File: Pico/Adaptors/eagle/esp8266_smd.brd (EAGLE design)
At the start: 29.5 x 17.8 mm, 3 parts

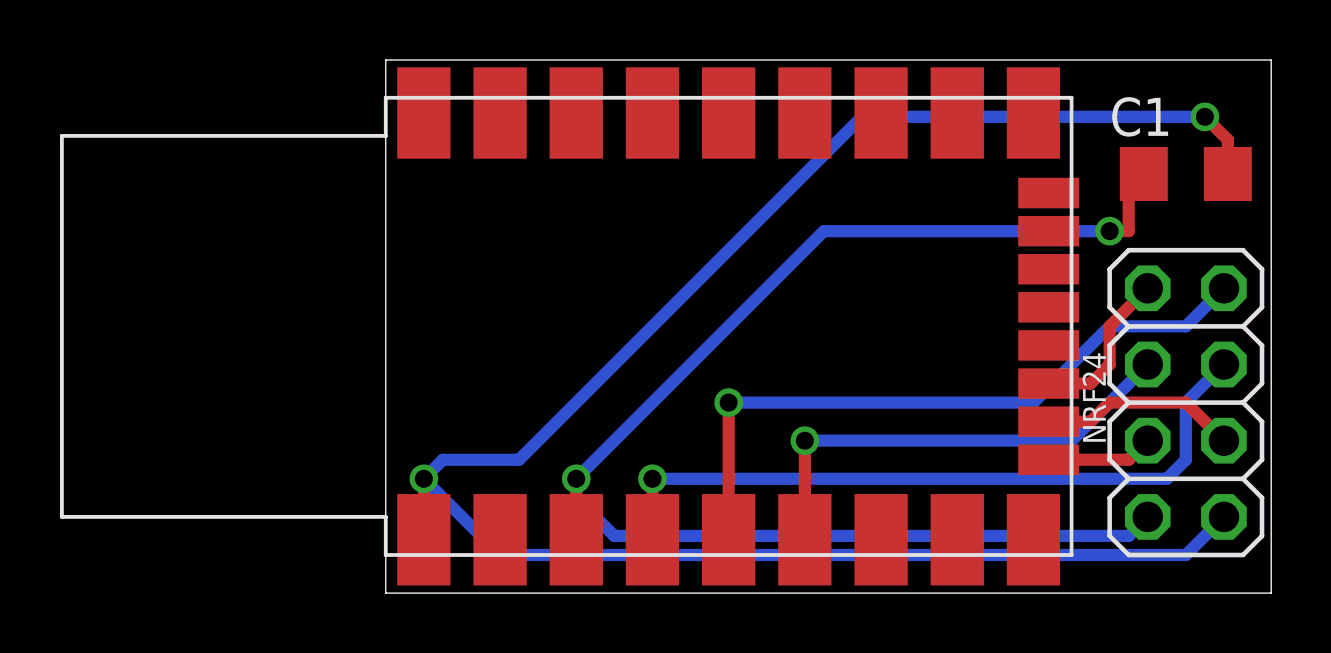
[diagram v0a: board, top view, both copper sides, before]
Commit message: tweaking
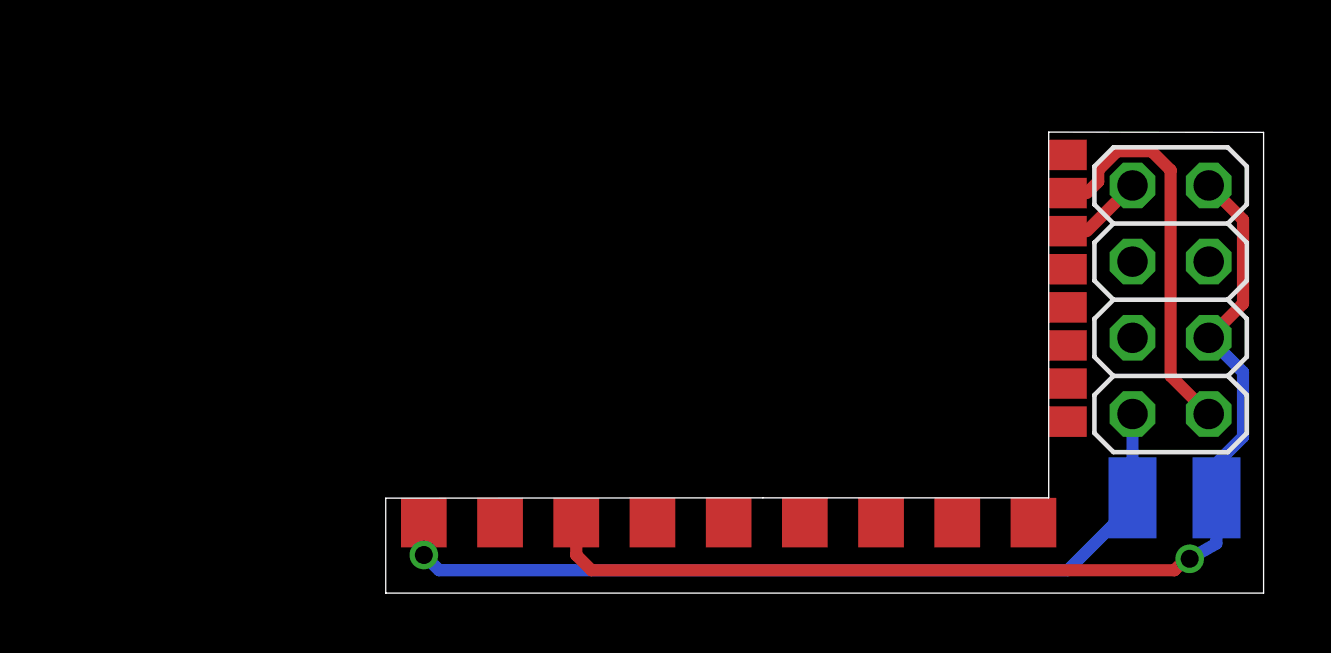
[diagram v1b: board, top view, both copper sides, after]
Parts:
- removed NRF24: (no value), pinhead:2X04
- removed U$1: ESPRUINO_PICO_SMDONLY, espruino_pico:ESPRUINO_PICO_SMDONLY
- added ESP8266: (no value), pinhead:2X04
- C1: device rcl:C1206 -> rcl:C1210
- moved C1 10.8 mm to (26.3, 3.17), flipped to the bottom
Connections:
- removed net N$1: C1.1, NRF24.2, U$1.3.3V
- removed net N$2: C1.2, NRF24.1, U$1.GND
- removed net N$4: NRF24.5, U$1.B3
- removed net N$5: NRF24.7, U$1.B4
- removed net N$6: NRF24.6, U$1.B5
- removed net N$7: NRF24.4, U$1.B8
- removed net N$8: NRF24.3, U$1.B9
- removed net N$9: NRF24.8, U$1.A10
- new net ESP_RX: ESP8266.1
- new net ESP_TX: ESP8266.8
- new net GND: C1.2, ESP8266.7
- new net VCC: C1.1, ESP8266.2, ESP8266.6
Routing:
- net N$2: track 63.5 -> 0.00 mm, vias 2 -> 0
- net N$1: track 46.5 -> 0.00 mm, vias 2 -> 0
- net VCC: track 0.00 -> 36.8 mm, vias 0 -> 1
- net GND: track 0.00 -> 28.7 mm, vias 0 -> 1
- net N$4: track 23.8 -> 0.00 mm, vias 1 -> 0
- net N$5: track 22.7 -> 0.00 mm, vias 1 -> 0
- net N$6: track 15.8 -> 0.00 mm, vias 1 -> 0
- net ESP_TX: track 0.00 -> 12.5 mm
- net N$8: track 6.63 -> 0.00 mm
- net N$9: track 5.36 -> 0.00 mm
- net N$7: track 3.57 -> 0.00 mm
- net ESP_RX: track 0.00 -> 2.16 mm
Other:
- board size 29.5 x 17.8 mm -> 29.3 x 15.4 mm
